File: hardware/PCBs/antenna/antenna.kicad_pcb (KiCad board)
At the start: 2 copper layers, 44 x 50 mm, 10 parts

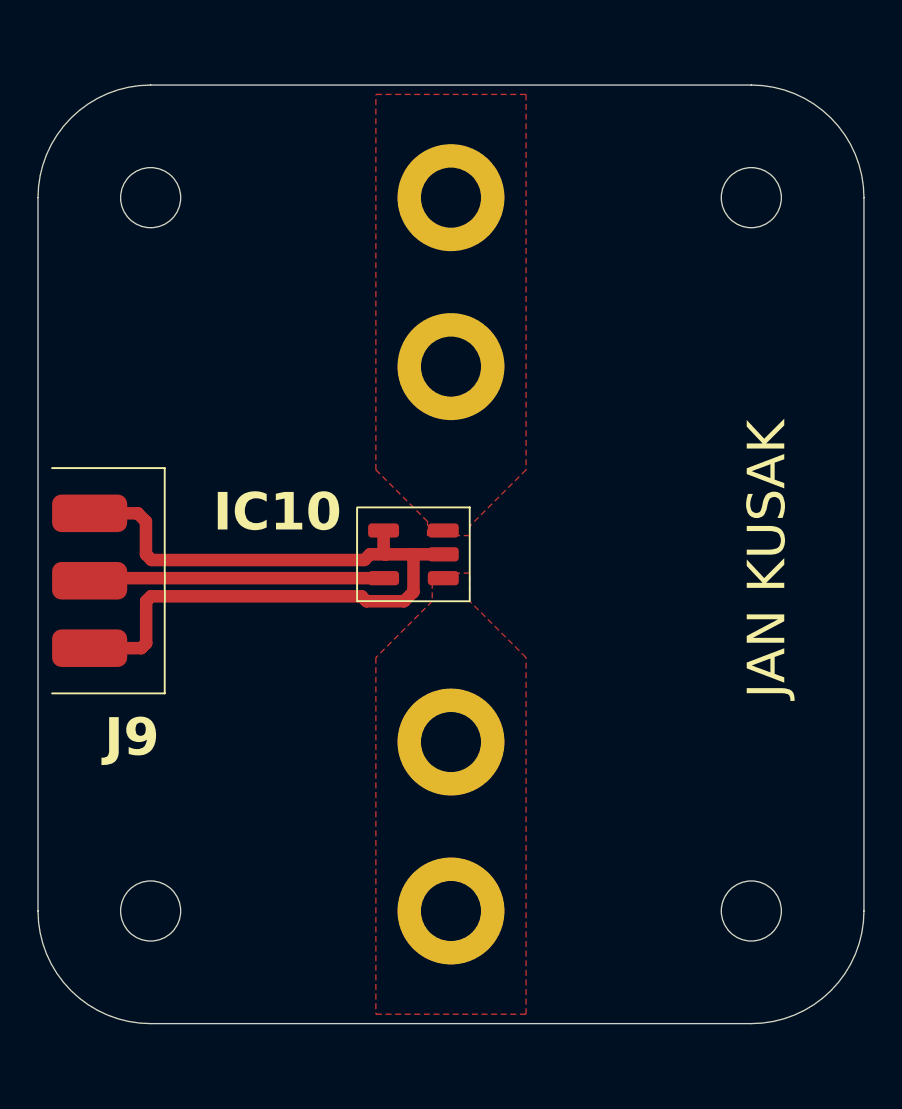
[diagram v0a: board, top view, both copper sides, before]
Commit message: Ant done
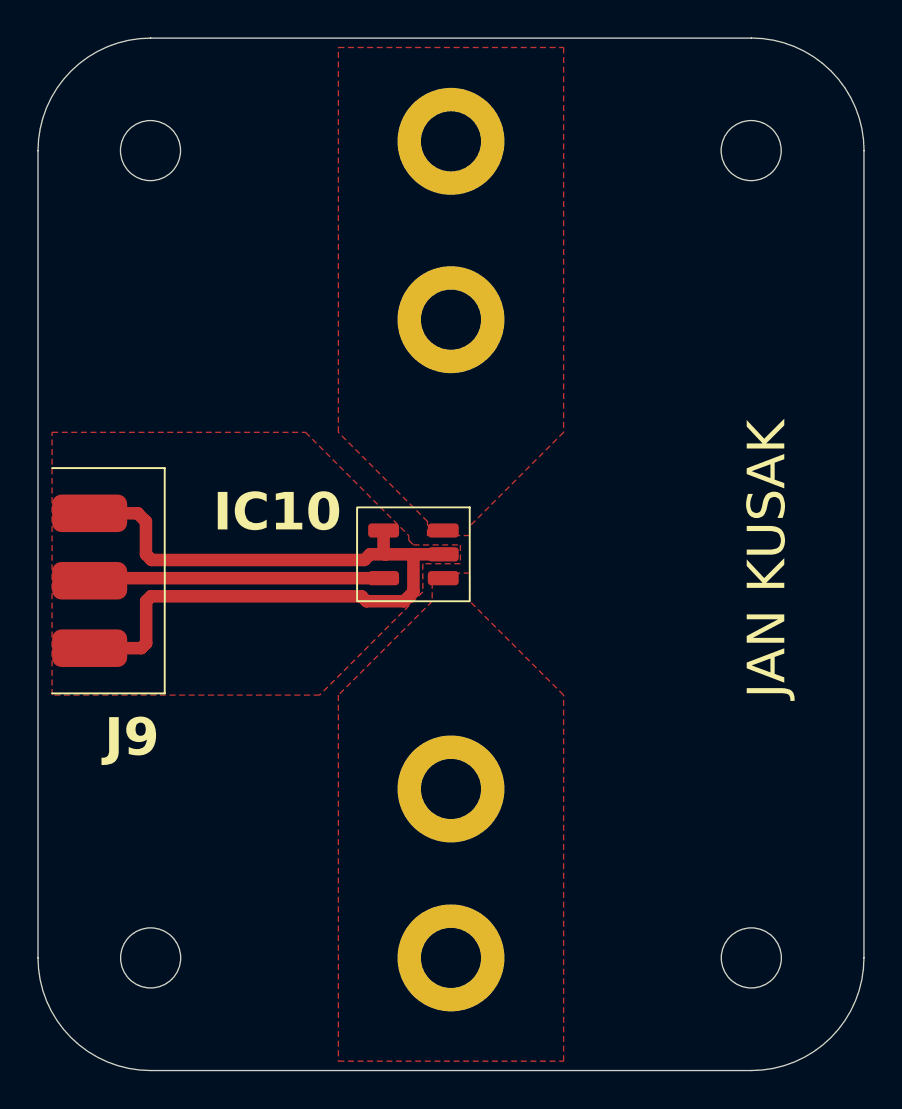
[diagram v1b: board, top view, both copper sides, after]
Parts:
- moved H1 3.00 mm to (128.0, 55.0)
- moved H5 2.51 mm to (112.0, 55.5)
- moved H6 2.51 mm to (144.0, 55.5)
- moved H 2.50 mm to (144.0, 98.5)
- moved H2 2.50 mm to (128.0, 64.5)
- moved H3 2.50 mm to (128.0, 89.5)
- moved H4 2.50 mm to (128.0, 98.5)
- moved H8 2.50 mm to (112.0, 98.5)
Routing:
- added copper zone on F.Cu, net GND
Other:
- board size 44 x 50 mm -> 44 x 55 mm
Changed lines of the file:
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@@
 		(allow_soldermask_bridges_in_footprints no)
 		(pcbplotparams
-			(layerselection 0x00010fc_ffffffff)
+			(layerselection 0x00010b8_ffffffff)
 			(plot_on_all_layers_selection 0x0000000_00000000)
 			(disableapertmacros no)
@@
 			(psnegative no)
 			(psa4output no)
-			(plotreference yes)
-			(plotvalue yes)
-			(plotfptext yes)
+			(plotreference no)
+			(plotvalue no)
+			(plotfptext no)
 			(plotinvisibletext no)
 			(sketchpadsonfab no)
 			(subtractmaskfromsilk no)
-			(outputformat 1)
+			(outputformat 4)
 			(mirror no)
-			(drillshape 1)
+			(drillshape 0)
 			(scaleselection 1)
-			(outputdirectory "")
+			(outputdirectory "gerber/")
 		)
 	)
@@
 	(footprint "MountingHole:MountingHole_3.2mm_M3_ISO7380_Pad"
 		(layer "F.Cu")
-		(at 128 58)
+		(at 128 55)
 		(descr "Mounting Hole 3.2mm, M3, ISO7380")
 		(tags "mounting hole 3.2mm m3 iso7380")
@@
 	(footprint "MountingHole:MountingHole_3.2mm_M3_ISO7380_Pad"
 		(layer "F.Cu")
-		(at 128 96)
+		(at 128 98.5)
 		(descr "Mounting Hole 3.2mm, M3, ISO7380")
 		(tags "mounting hole 3.2mm m3 iso7380")
@@
 	(footprint "MountingHole:MountingHole_3.2mm_M3"
 		(layer "F.Cu")
-		(at 112 96)
+		(at 112 98.5)
 		(descr "Mounting Hole 3.2mm, no annular, M3")
 		(tags "mounting hole 3.2mm no annular m3")
@@
 	(footprint "MountingHole:MountingHole_3.2mm_M3_ISO7380_Pad"
 		(layer "F.Cu")
-		(at 128 67)
+		(at 128 64.5)
 		(descr "Mounting Hole 3.2mm, M3, ISO7380")
 		(tags "mounting hole 3.2mm m3 iso7380")
@@
 	(footprint "MountingHole:MountingHole_3.2mm_M3_ISO7380_Pad"
 		(layer "F.Cu")
-		(at 128 87)
+		(at 128 89.5)
 		(descr "Mounting Hole 3.2mm, M3, ISO7380")
 		(tags "mounting hole 3.2mm m3 iso7380")
@@
 	(footprint "MountingHole:MountingHole_3.2mm_M3"
 		(layer "F.Cu")
-		(at 144 96)
+		(at 144 98.5)
 		(descr "Mounting Hole 3.2mm, no annular, M3")
 		(tags "mounting hole 3.2mm no annular m3")
@@
 	(footprint "MountingHole:MountingHole_3.2mm_M3"
 		(layer "F.Cu")
-		(at 112 58)
+		(at 111.992641 55.492641)
 		(descr "Mounting Hole 3.2mm, no annular, M3")
 		(tags "mounting hole 3.2mm no annular m3")
@@
 	(footprint "MountingHole:MountingHole_3.2mm_M3"
 		(layer "F.Cu")
-		(at 144 58)
+		(at 143.992641 55.492641)
 		(descr "Mounting Hole 3.2mm, no annular, M3")
 		(tags "mounting hole 3.2mm no annular m3")
@@
 	)
 	(gr_arc
-		(start 112 102)
-		(mid 107.757359 100.242641)
-		(end 106 96)
+		(start 112 104.5)
+		(mid 107.757359 102.742641)
+		(end 106 98.5)
 		(stroke
 			(width 0.05)
@@
 	)
 	(gr_line
-		(start 150 58)
-		(end 150 96)
+		(start 150 55.5)
+		(end 150 98.5)
 		(stroke
 			(width 0.05)
@@
 	)
 	(gr_line
-		(start 144 102)
-		(end 112 102)
+		(start 144 104.5)
+		(end 112 104.5)
 		(stroke
 			(width 0.05)
@@
 		(layer "Edge.Cuts")
 	)
-	(gr_line
-		(start 112 52)
-		(end 144 52)
+	(gr_arc
+		(start 144 49.494794)
+		(mid 148.246322 51.253678)
+		(end 150.005206 55.5)
 		(stroke
 			(width 0.05)
@@
 		(layer "Edge.Cuts")
 	)
-	(gr_line
-		(start 106 96)
-		(end 106 58)
+	(gr_arc
+		(start 150 98.5)
+		(mid 148.242641 102.742641)
+		(end 144 104.5)
 		(stroke
 			(width 0.05)
@@
 	)
 	(gr_arc
-		(start 106 58)
-		(mid 107.757359 53.757359)
-		(end 112 52)
+		(start 105.999996 55.5)
+		(mid 107.757356 51.257356)
+		(end 112 49.499996)
 		(stroke
 			(width 0.05)
@@
 		(layer "Edge.Cuts")
 	)
-	(gr_arc
-		(start 144 52)
-		(mid 148.242641 53.757359)
-		(end 150 58)
+	(gr_line
+		(start 111.992641 49.5)
+		(end 143.992641 49.5)
 		(stroke
 			(width 0.05)
@@
 		(layer "Edge.Cuts")
 	)
-	(gr_arc
-		(start 150 96)
-		(mid 148.242641 100.242641)
-		(end 144 102)
+	(gr_line
+		(start 106 98.5)
+		(end 106 55.5)
 		(stroke
 			(width 0.05)
@@
 		(layer "F.Cu")
 		(hatch full 0.6)
-		(priority 1)
+		(priority 2)
 		(connect_pads yes
 			(clearance 0.6)
@@
 		(polygon
 			(pts
-				(xy 127 78) (xy 127 79.5) (xy 124 82.5) (xy 124 101.5) (xy 132 101.5) (xy 132 82.5) (xy 129 79.5)
-				(xy 129 78)
+				(xy 127 78) (xy 127 79.5) (xy 122 84.5) (xy 122 104) (xy 134 104) (xy 134 84.5) (xy 129 79.5) (xy 129 78)
+			)
+		)
+	)
+	(zone
+		(net 2)
+		(net_name "GND")
+		(layer "F.Cu")
+		(hatch edge 0.5)
+		(connect_pads yes
+			(clearance 0.3)
+		)
+		(min_thickness 0.25)
+		(filled_areas_thickness no)
+		(fill yes
+			(thermal_gap 0.5)
+			(thermal_bridge_width 0.5)
+			(smoothing fillet)
+			(radius 1)
+		)
+		(polygon
+			(pts
+				(xy 106.75 70.5) (xy 120.25 70.5) (xy 125.75 76) (xy 125.75 76.25) (xy 126 76.5) (xy 128.5 76.5)
+				(xy 128.5 77.5) (xy 126.5 77.5) (xy 126.5 79) (xy 121 84.5) (xy 106.75 84.5)
 			)
 		)
@@
 		(layer "F.Cu")
 		(hatch edge 0.5)
+		(priority 2)
 		(connect_pads yes
 			(clearance 0.6)
@@
 		(polygon
 			(pts
-				(xy 124 52.5) (xy 132 52.5) (xy 132 72.5) (xy 129 75.5) (xy 129 76) (xy 126.75 76) (xy 126.75 75.25)
-				(xy 124 72.5)
+				(xy 122 50) (xy 134 50) (xy 134 70.5) (xy 129 75.5) (xy 129 76) (xy 126.75 76) (xy 126.75 75.25)
+				(xy 122 70.5)
 			)
 		)
@@
 		(polygon
 			(pts
-				(xy 124 52.5) (xy 132 52.5) (xy 132 72.5) (xy 129 72.5) (xy 126.5 72.5) (xy 124 72.5)
+				(xy 122 50) (xy 134 50) (xy 134 70.5) (xy 129.25 70.5) (xy 126.75 70.5) (xy 122 70.5)
 			)
 		)
@@
 		(polygon
 			(pts
-				(xy 124 82.5) (xy 132 82.5) (xy 132 101.5) (xy 124 101.5)
-			)
-		)
+				(xy 122 84.5) (xy 134 84.5) (xy 134 104) (xy 122 104)
+			)
+		)
